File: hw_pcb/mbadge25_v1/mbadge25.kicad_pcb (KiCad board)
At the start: 2 copper layers, 8 parts, among them J1 USB4105-GF-A, U1 ESP32-C3-MINI-1

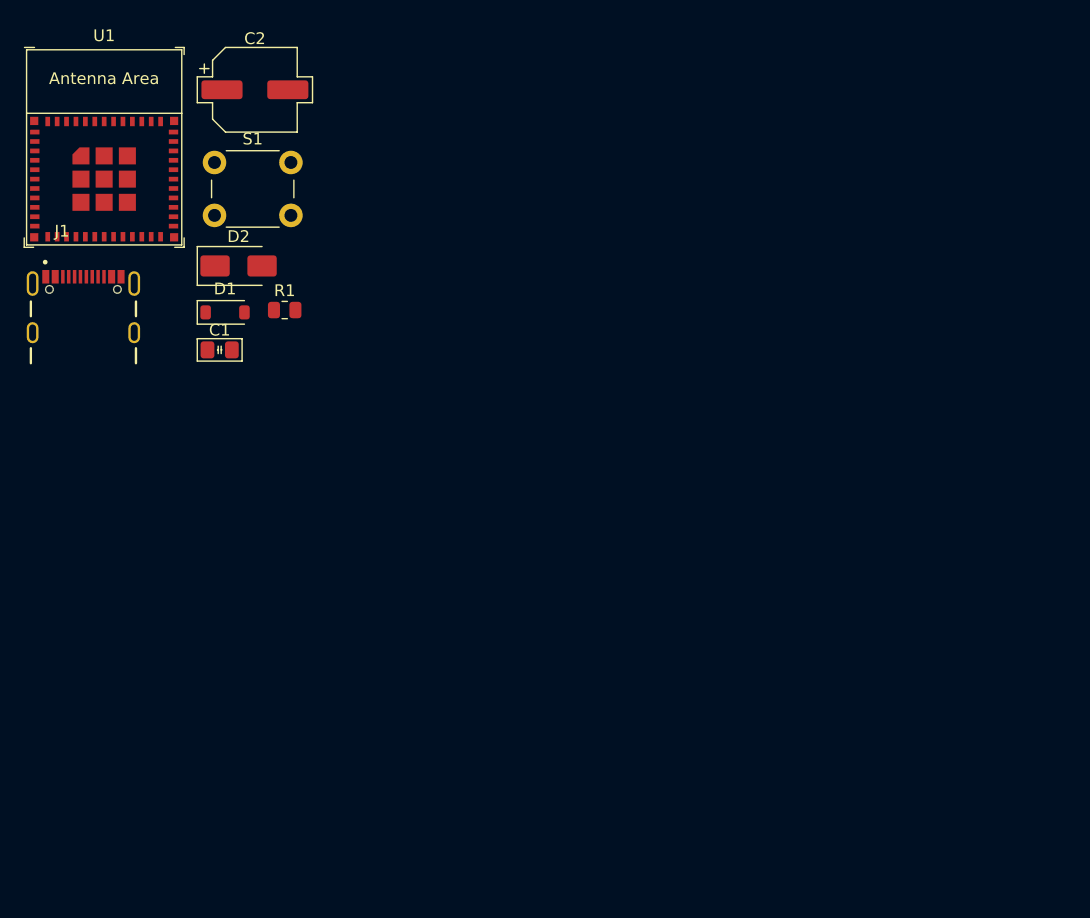
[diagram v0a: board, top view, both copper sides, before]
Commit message: v1 draft PCB layout
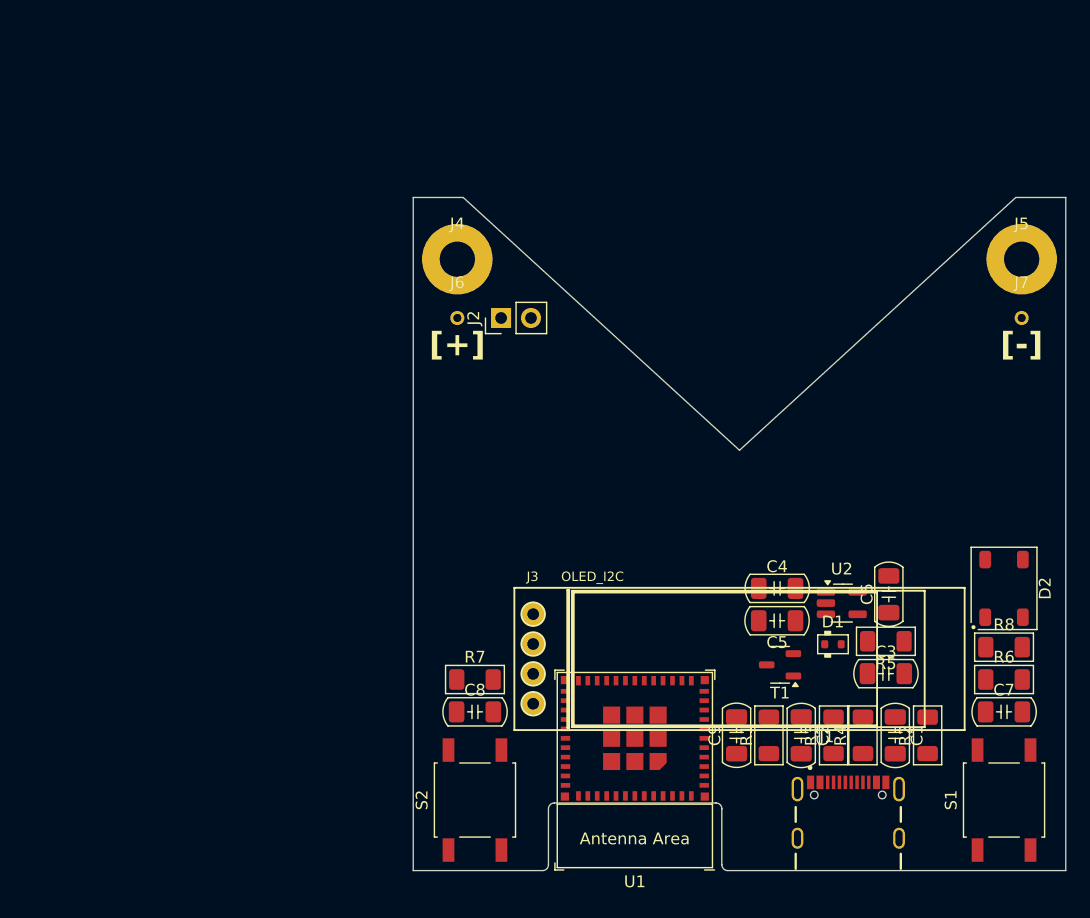
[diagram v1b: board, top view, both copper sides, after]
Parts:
- added C3: 100nF, Library_FP_mbadge25:C_1206_3216Metric_Pad1.33x1.80mm, F.Cu at (112.5, 83.2)
- added C4: 2.2µF, Library_FP_mbadge25:C_1206_3216Metric_Pad1.33x1.80mm, F.Cu at (103.2, 76.0)
- added C5: 2.2µF, Library_FP_mbadge25:C_1206_3216Metric_Pad1.33x1.80mm, F.Cu at (103.2, 78.8)
- added C6: 2.2µF, Library_FP_mbadge25:C_1206_3216Metric_Pad1.33x1.80mm, F.Cu at (112.7, 76.5)
- added C7: 100nF, Library_FP_mbadge25:C_1206_3216Metric_Pad1.33x1.80mm, F.Cu at (122.5, 86.5)
- added C8: 1µF, Library_FP_mbadge25:C_1206_3216Metric_Pad1.33x1.80mm, F.Cu at (77.5, 86.5)
- added C9: 1µF, Library_FP_mbadge25:C_1206_3216Metric_Pad1.33x1.80mm, F.Cu at (99.8, 88.5)
- added J2: BAT, Library_FP_mbadge25:PinHeader_1x02_P2.54mm_Vertical, F.Cu at (79.7, 53.0)
- added J3: OLED_I2C, Library_FP_mbadge25:OLED_128x32, F.Cu at (100.0, 82.0)
- added J4: BAT, Library_FP_mbadge25:Pad_6.0mm_Drill3.0mm, F.Cu at (76.0, 48.0)
- added J5: GND, Library_FP_mbadge25:Pad_6.0mm_Drill3.0mm, F.Cu at (124.0, 48.0)
- added J6: BAT, Library_FP_mbadge25:Pad_1.2mm_Drill0.7mm, F.Cu at (76.0, 53.0)
- added J7: GND, Library_FP_mbadge25:Pad_1.2mm_Drill0.7mm, F.Cu at (124.0, 53.0)
- added R2: 5k1, Library_FP_mbadge25:R_1206_3216Metric_Pad1.30x1.75mm, F.Cu at (116.0, 88.5)
- added R3: 27E, Library_FP_mbadge25:R_1206_3216Metric_Pad1.30x1.75mm, F.Cu at (108.0, 88.5)
- added R4: 27E, Library_FP_mbadge25:R_1206_3216Metric_Pad1.30x1.75mm, F.Cu at (110.5, 88.5)
- added R5: 100k, Library_FP_mbadge25:R_1206_3216Metric_Pad1.30x1.75mm, F.Cu at (112.5, 80.5)
- added R6: 100k, Library_FP_mbadge25:R_1206_3216Metric_Pad1.30x1.75mm, F.Cu at (122.5, 83.8)
- added R7: 10k, Library_FP_mbadge25:R_1206_3216Metric_Pad1.30x1.75mm, F.Cu at (77.5, 83.8)
- added R8: 220E, Library_FP_mbadge25:R_1206_3216Metric_Pad1.30x1.75mm, F.Cu at (122.5, 81.0)
- added S2: RST, Library_FP_mbadge25:SW_SPST, F.Cu at (77.5, 94.0)
- added T1: LP0404N3T5G, Library_FP_mbadge25:SOT-23-3, F.Cu at (103.5, 82.5)
- added U2: XC6220B331MR, Library_FP_mbadge25:SOT-23-5_HandSoldering, F.Cu at (108.7, 77.2)
- C1: value C -> 47pF; footprint PCM_Capacitor_SMD_AKL:C_0805_2012Metric_Pad1.18x1.45mm_HandSolder -> Library_FP_mbadge25:C_1206_3216Metric_Pad1.33x1.80mm
- C2: value C-polar -> 47pF; footprint PCM_Capacitor_SMD_AKL:CP_Elec_6.3x5.9 -> Library_FP_mbadge25:C_1206_3216Metric_Pad1.33x1.80mm
- D1: value type="" model="D" lib="semiconductor.lib" -> MSK4005; footprint Diode_SMD:D_SOD-123 -> Library_FP_mbadge25:D_SOD-523
- D2: value type="" model="D-LED" lib="semiconductor.lib" -> WS2812B; footprint Diode_SMD:D_SMA -> Library_FP_mbadge25:LED_WS2812B_PLCC4_5.0x5.0mm_P3.2mm
- R1: value R -> 5k1; footprint Resistor_SMD:R_0805_2012Metric -> Library_FP_mbadge25:R_1206_3216Metric_Pad1.30x1.75mm
- S1: value S-make-push -> SW; footprint Button_Switch_THT:SW_PUSH_6mm -> Library_FP_mbadge25:SW_SPST
- U1: footprint PCM_Espressif:ESP32-C3-MINI-1 -> Library_FP_mbadge25:ESP32-C3-MINI-1
- moved S1 86.3 mm to (122.5, 94.0), turned to 90 degrees
- moved J1 78.0 mm to (109.2, 97.2)
- moved C2 71.9 mm to (105.2, 88.5), turned to -90 degrees
- moved D2 70.6 mm to (122.5, 76.0), turned to -90 degrees
- moved U1 69.6 mm to (91.1, 91.5), turned to 180 degrees
- moved C1 66.2 mm to (113.2, 88.5), turned to -90 degrees
- moved D1 58.9 mm to (108.0, 80.8)
- moved R1 54.8 mm to (102.5, 88.5), turned to 90 degrees
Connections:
- C1 pad 1: unconnected-(C1-+-Pad1) -> /IO18.USBN
- C1 pad 2: unconnected-(C1---Pad2) -> /GND
- C2 pad 1: unconnected-(C2-+-Pad1) -> /IO19.USBP
- C2 pad 2: unconnected-(C2---Pad2) -> /GND
- D1 pad 1: unconnected-(D1-K--Pad1) -> /5V0
- D1 pad 2: unconnected-(D1-A+-Pad2) -> /VUSB
- D2 pad 1: unconnected-(D2-K--Pad1) -> /5V0
- D2 pad 2: unconnected-(D2-A+-Pad2) -> /RGB.DO
- J1 pad A1_B12: unconnected-(J1-GND-PadA1_B12) -> /GND
- J1 pad A4_B9: unconnected-(J1-VBUS-PadA4_B9) -> /VUSB
- J1 pad A5: unconnected-(J1-CC1-PadA5) -> Net-(J1-CC1)
- J1 pad A6: unconnected-(J1-DP1-PadA6) -> /DP
- J1 pad A7: unconnected-(J1-DN1-PadA7) -> /DN
- J1 pad B1_A12: unconnected-(J1-GND__1-PadB1_A12) -> /GND
- J1 pad B4_A9: unconnected-(J1-VBUS__1-PadB4_A9) -> /VUSB
- J1 pad B5: unconnected-(J1-CC2-PadB5) -> Net-(J1-CC2)
- J1 pad B6: unconnected-(J1-DP2-PadB6) -> /DP
- J1 pad B7: unconnected-(J1-DN2-PadB7) -> /DN
- J1 pad SH1: unconnected-(J1-SHELL_GND-PadSH1) -> /GND
- J1 pad SH2: unconnected-(J1-SHELL_GND__1-PadSH2) -> /GND
- J1 pad SH3: unconnected-(J1-SHELL_GND__2-PadSH3) -> /GND
- J1 pad SH4: unconnected-(J1-SHELL_GND__3-PadSH4) -> /GND
- R1 pad 1: unconnected-(R1-+-Pad1) -> Net-(J1-CC1)
- R1 pad 2: unconnected-(R1---Pad2) -> /GND
- S1 pad 1: (no net) -> /IO9
- S1 pad 2: (no net) -> /GND
- U1 pad 1: Net-(U1-GND-Pad1) -> /GND
- U1 pad 11: Net-(U1-GND-Pad1) -> /GND
- U1 pad 14: Net-(U1-GND-Pad1) -> /GND
- U1 pad 16: unconnected-(U1-GPIO10-Pad16) -> /IO10
- U1 pad 18: unconnected-(U1-GPIO4/ADC1_CH4-Pad18) -> /IO4
- U1 pad 19: unconnected-(U1-GPIO5/ADC2_CH0-Pad19) -> /IO5
- U1 pad 2: Net-(U1-GND-Pad1) -> /GND
- U1 pad 20: unconnected-(U1-GPIO6-Pad20) -> /IO6.RGB
- U1 pad 21: unconnected-(U1-GPIO7-Pad21) -> /IO7.SDA
- U1 pad 22: unconnected-(U1-GPIO8-Pad22) -> /IO8.SCL
- U1 pad 23: unconnected-(U1-GPIO9-Pad23) -> /IO9
- U1 pad 26: unconnected-(U1-GPIO18/USB_D--Pad26) -> /IO18.USBN
- U1 pad 27: unconnected-(U1-GPIO19/USB_D+-Pad27) -> /IO19.USBP
- U1 pad 3: unconnected-(U1-3V3-Pad3) -> /3V3
- U1 pad 30: unconnected-(U1-GPIO20/U0RXD-Pad30) -> /IO20.RX
- U1 pad 31: unconnected-(U1-GPIO21/U0TXD-Pad31) -> /IO21.TX
- U1 pad 36: Net-(U1-GND-Pad1) -> /GND
- U1 pad 37: Net-(U1-GND-Pad1) -> /GND
- U1 pad 38: Net-(U1-GND-Pad1) -> /GND
- U1 pad 39: Net-(U1-GND-Pad1) -> /GND
- U1 pad 40: Net-(U1-GND-Pad1) -> /GND
- U1 pad 41: Net-(U1-GND-Pad1) -> /GND
- U1 pad 42: Net-(U1-GND-Pad1) -> /GND
- U1 pad 43: Net-(U1-GND-Pad1) -> /GND
- U1 pad 44: Net-(U1-GND-Pad1) -> /GND
- U1 pad 45: Net-(U1-GND-Pad1) -> /GND
- U1 pad 46: Net-(U1-GND-Pad1) -> /GND
- U1 pad 47: Net-(U1-GND-Pad1) -> /GND
- U1 pad 48: Net-(U1-GND-Pad1) -> /GND
- U1 pad 49: Net-(U1-GND-Pad1) -> /GND
- U1 pad 5: unconnected-(U1-GPIO2/ADC1_CH2-Pad5) -> /IO2
- U1 pad 50: Net-(U1-GND-Pad1) -> /GND
- U1 pad 51: Net-(U1-GND-Pad1) -> /GND
- U1 pad 52: Net-(U1-GND-Pad1) -> /GND
- U1 pad 53: Net-(U1-GND-Pad1) -> /GND
- U1 pad 6: unconnected-(U1-GPIO3/ADC1_CH3-Pad6) -> /IO3
- U1 pad 8: unconnected-(U1-EN/CHIP_PU-Pad8) -> Net-(C8-+)
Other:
- board outline added: 55.5 x 57.2 mm
- board text added: "[+]"
- board text added: "[-]"

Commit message: v2 draft PCB layout
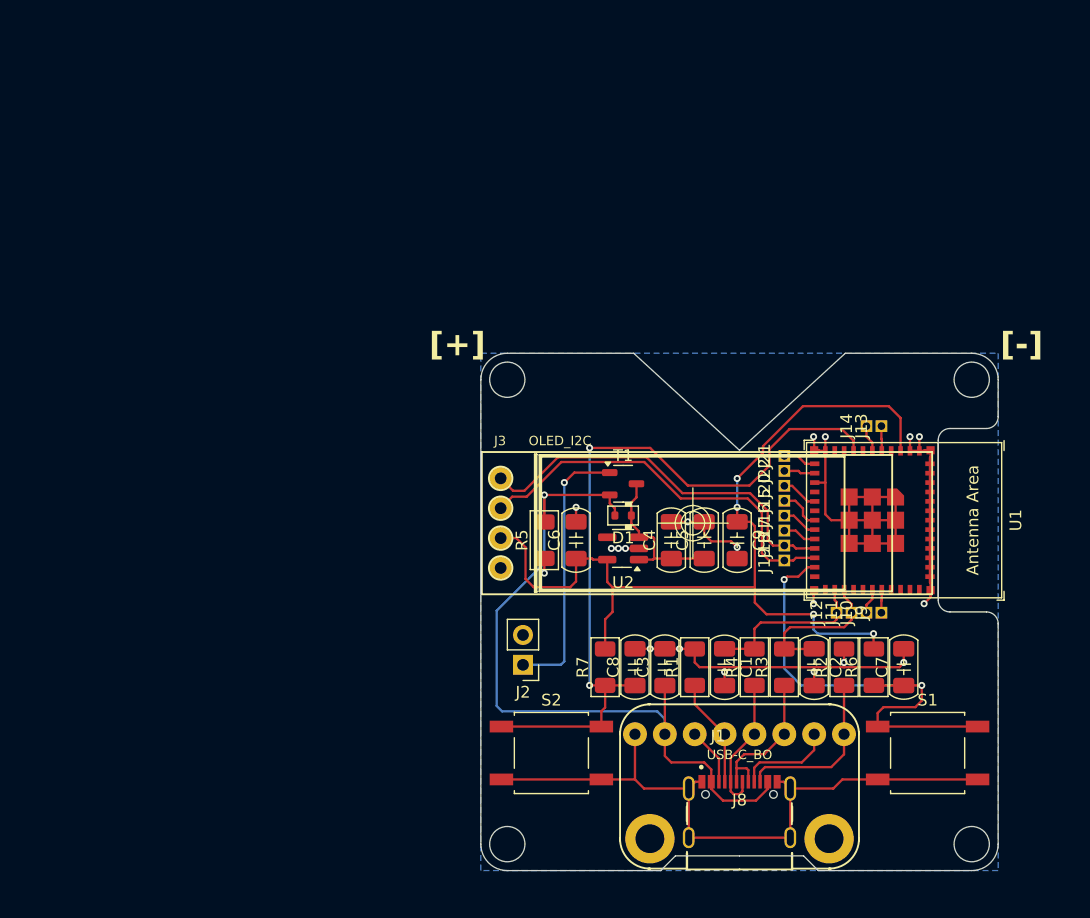
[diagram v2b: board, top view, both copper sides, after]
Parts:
- removed D2: WS2812B, Library_FP_mbadge25:LED_WS2812B_PLCC4_5.0x5.0mm_P3.2mm
- removed J4: BAT, Library_FP_mbadge25:Pad_6.0mm_Drill3.0mm
- removed J5: GND, Library_FP_mbadge25:Pad_6.0mm_Drill3.0mm
- removed J6: BAT, Library_FP_mbadge25:Pad_1.2mm_Drill0.7mm
- removed J7: GND, Library_FP_mbadge25:Pad_1.2mm_Drill0.7mm
- removed R8: 220E, Library_FP_mbadge25:R_1206_3216Metric_Pad1.30x1.75mm
- added J10: Conn_IO20.RX, Library_FP_mbadge25:PinHeader_1x01_P1.27mm_Vertical, F.Cu at (110.8, 78.1)
- added J11: Conn_IO19.USBP, Library_FP_mbadge25:PinHeader_1x01_P1.27mm_Vertical, F.Cu at (109.5, 78.1)
- added J12: Conn_IO18.USBN, Library_FP_mbadge25:PinHeader_1x01_P1.27mm_Vertical, F.Cu at (108.3, 78.1)
- added J13: Conn_IO2, Library_FP_mbadge25:PinHeader_1x01_P1.27mm_Vertical, F.Cu at (112.1, 62.2)
- added J14: Conn_IO3, Library_FP_mbadge25:PinHeader_1x01_P1.27mm_Vertical, F.Cu at (110.8, 62.2)
- added J15: Conn_IO4, Library_FP_mbadge25:PinHeader_1x01_P1.27mm_Vertical, F.Cu at (103.8, 68.5)
- added J16: Conn_IO5, Library_FP_mbadge25:PinHeader_1x01_P1.27mm_Vertical, F.Cu at (103.8, 69.8)
- added J17: Conn_IO6.RGB, Library_FP_mbadge25:PinHeader_1x01_P1.27mm_Vertical, F.Cu at (103.8, 71.1)
- added J18: Conn_IO7.SDA, Library_FP_mbadge25:PinHeader_1x01_P1.27mm_Vertical, F.Cu at (103.8, 72.4)
- added J19: Conn_IO8.SCL, Library_FP_mbadge25:PinHeader_1x01_P1.27mm_Vertical, F.Cu at (103.8, 73.6)
- added J20: Conn_IO10, Library_FP_mbadge25:PinHeader_1x01_P1.27mm_Vertical, F.Cu at (103.8, 67.3)
- added J21: Conn_IO00, Library_FP_mbadge25:PinHeader_1x01_P1.27mm_Vertical, F.Cu at (103.8, 64.7)
- added J22: Conn_IO01, Library_FP_mbadge25:PinHeader_1x01_P1.27mm_Vertical, F.Cu at (103.8, 66.0)
- added J8: USB-C_BO, Library_FP_mbadge25:USB_C_BO, F.Cu at (100.0, 88.4)
- added J9: Conn_IO21.TX, Library_FP_mbadge25:PinHeader_1x01_P1.27mm_Vertical, F.Cu at (112.1, 78.1)
- moved U1 31.2 mm to (114.0, 70.2), turned to -90 degrees
- moved R5 30.3 mm to (83.4, 71.9), turned to 90 degrees
- moved J2 29.6 mm to (81.6, 82.5), turned to 180 degrees
- moved C6 27.0 mm to (86.1, 71.9)
- moved D1 20.9 mm to (90.1, 69.8), turned to 180 degrees
- moved T1 20.4 mm to (90.1, 67.1), turned to 0 degrees
- moved U2 19.2 mm to (90.1, 72.6), turned to 180 degrees
- moved C3 18.8 mm to (93.7, 82.7), turned to 90 degrees
- moved C9 16.6 mm to (99.8, 71.9), turned to -90 degrees
- moved C1 15.6 mm to (98.7, 82.7)
- moved C8 14.1 mm to (91.1, 82.7), turned to 90 degrees
- moved J3 11.9 mm to (97.2, 70.5)
- moved R6 11.1 mm to (111.4, 82.7), turned to 90 degrees
- moved R7 11.1 mm to (88.6, 82.7), turned to 90 degrees
- moved R4 10.9 mm to (101.3, 82.7)
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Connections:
- net /IO9 renamed /IO9.SW
- net Net-(C8-+) renamed /EN
- net Net-(J1-CC1) renamed /CC1
- net Net-(J1-CC2) renamed /CC2
- J1 pad A8: unconnected-(J1-SBU1-PadA8) -> /SBU1
- J1 pad B8: unconnected-(J1-SBU2-PadB8) -> /SBU2
- U1 pad 12: unconnected-(U1-GPIO0/ADC1_CH0/XTAL_32K_P-Pad12) -> Net-(J21-Pin_1)
- U1 pad 13: unconnected-(U1-GPIO1/ADC1_CH1/XTAL_32K_N-Pad13) -> Net-(J22-Pin_1)
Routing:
- net /GND: track 0.00 -> 153.4 mm, vias 0 -> 19
- net /3V3: track 0.00 -> 79.8 mm, vias 0 -> 4
- net /EN: track 0.00 -> 64.0 mm, vias 0 -> 2
- net /VUSB: track 0.00 -> 63.8 mm, vias 0 -> 1
- net /IO9.SW: track 0.00 -> 42.1 mm, vias 0 -> 2
- net /IO8.SCL: track 0.00 -> 33.9 mm
- net /IO7.SDA: track 0.00 -> 33.0 mm
- net /VBAT: track 0.00 -> 23.1 mm, vias 0 -> 1
- net /CC2: track 0.00 -> 14.5 mm
- net /IO18.USBN: track 0.00 -> 14.2 mm
- net /5V0: track 0.00 -> 13.6 mm
- net /DP: track 0.00 -> 12.9 mm
- net /IO19.USBP: track 0.00 -> 12.9 mm
- net /DN: track 0.00 -> 11.8 mm
- net /CC1: track 0.00 -> 9.26 mm
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- added copper zone on B.Cu, net /GND
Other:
- board size 55.5 x 57.2 mm -> 44 x 44 mm
